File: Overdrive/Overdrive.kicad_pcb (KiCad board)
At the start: 2 copper layers, 60 x 110 mm, 50 parts, among them J1 IN, J2 DC IN, J3 OUT, Q1 MMBT2222A, Q2 MMBT2222A, SW1 SW_SPDT, U1 TL072

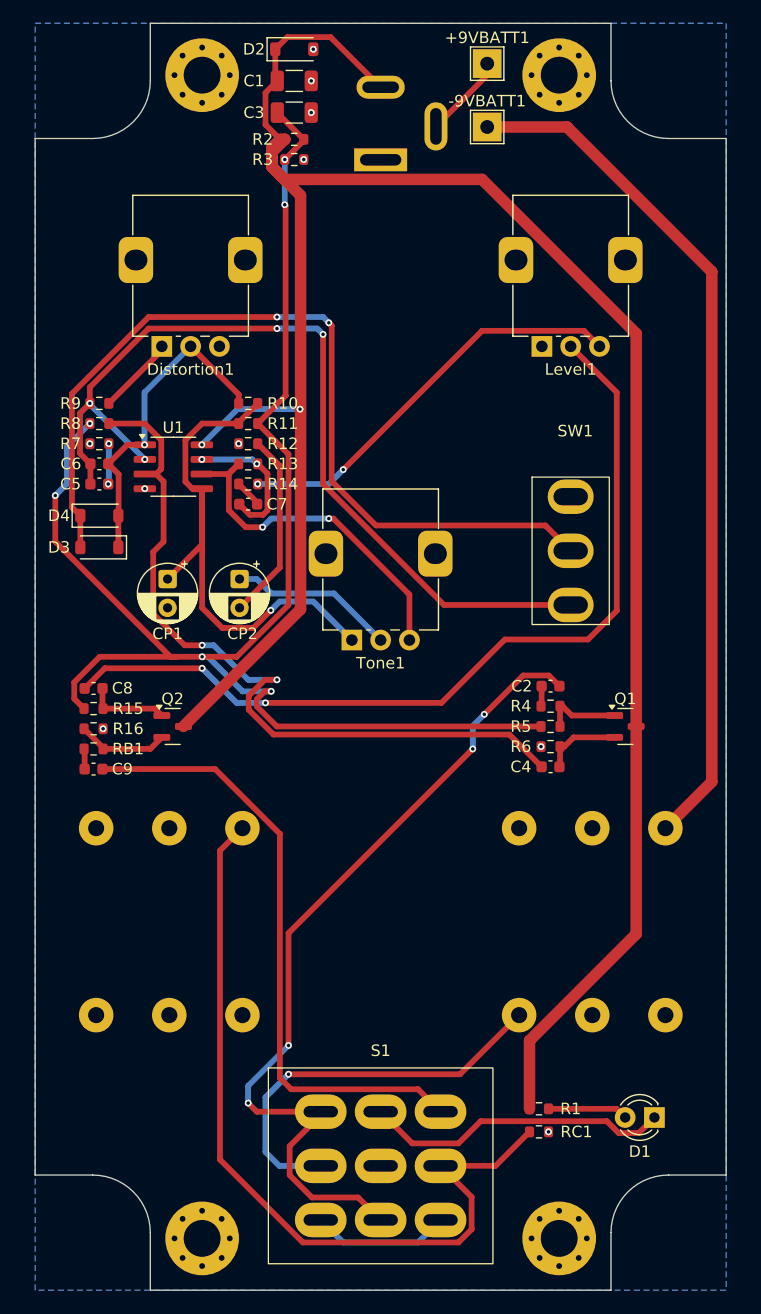
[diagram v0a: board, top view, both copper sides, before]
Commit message: done PCB layout
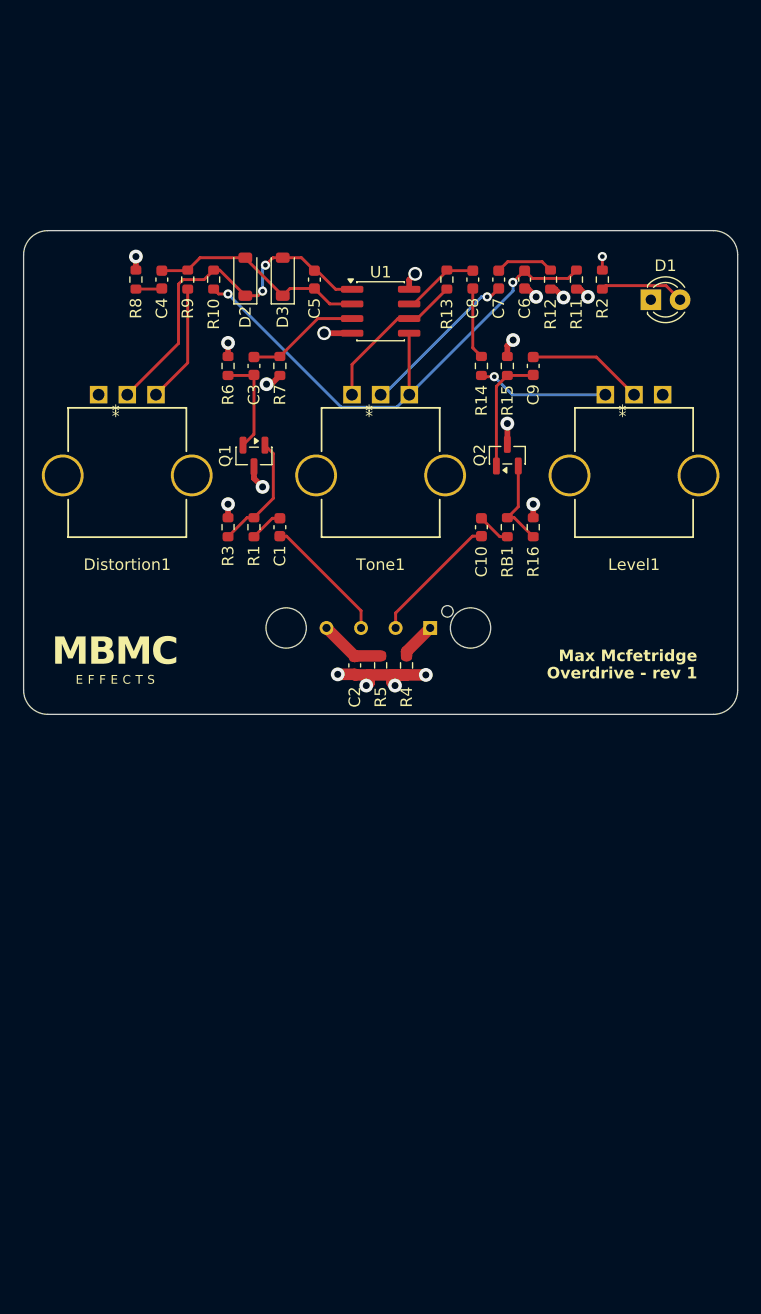
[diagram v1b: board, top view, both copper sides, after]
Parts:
- removed +9VBATT1: 9V Batt +ve, TestPoint:TestPoint_THTPad_2.5x2.5mm_Drill1.2mm
- removed -9VBATT1: 9V Batt -ve, TestPoint:TestPoint_THTPad_2.5x2.5mm_Drill1.2mm
- removed CP1, CP2: 220nF, Capacitor_THT:CP_Radial_D5.0mm_P2.50mm
- removed D4: 1N4148W, Diode_SMD:D_SOD-123
- removed H1, H2, H3, H4: MountingHole, MountingHole:MountingHole_3.2mm_M3_Pad_Via
- removed J2: DC IN, Connector_BarrelJack:BarrelJack_GCT_DCJ200-10-A_Horizontal
- removed J3: OUT, Connector_Audio:Jack_6.35mm_Neutrik_NMJ6HFD2_Horizontal
- removed RC1: 10k, Resistor_SMD:R_0603_1608Metric
- removed S1: Foot Switch, Button_Switch_THT:3PDT Foot Switch
- removed SW1: SW_SPDT, Button_Switch_THT:spdt switch custom
- added C10: 10uF, Capacitor_SMD:C_0603_1608Metric, F.Cu at (158.8, 83.8)
- C1: value 100uF -> 20nF; footprint Capacitor_SMD:C_1206_3216Metric -> Capacitor_SMD:C_0603_1608Metric
- C2: value 20nF -> 47uF
- C3: value 47uF -> 1uF; footprint Capacitor_SMD:C_1206_3216Metric -> Capacitor_SMD:C_0603_1608Metric
- C4: value 1uF -> 47nF
- C5: value 47nF -> 47pF
- C6: value 47pF -> 220nF
- C7: value 1uF -> 220nF
- C8: value 100nF -> 1uF
- C9: value 10uF -> 100nF
- Distortion1, Level1, Tone1: footprint Potentiometer_THT:Potentiometer_RK097_Single_Vertical -> PTV09A-4020F-A504:POT_PTV09A-4020F_BRN
- J1: value IN -> 303C-321018-30-04; footprint Connector_Audio:Jack_6.35mm_Neutrik_NMJ6HFD2_Horizontal -> 303C-321018-30-04:ATTEND_303C-321018-30-04
- R1: value 470R -> 1k
- R12: value 220 -> 220R
- R2: value 10K -> 470R
- R3: value 10K -> 510k
- R4: value 1k -> 10K
- R5: value 510k -> 10K
- R7: value 4.7k -> 10k
- R8: value 10k -> 4.7k
- moved D1 71.0 mm to (173.5, 64.0), turned to 0 degrees
- moved R1 56.2 mm to (139.0, 83.8), turned to 90 degrees
- moved C4 54.1 mm to (131.0, 62.2), turned to 90 degrees
- moved C9 51.8 mm to (163.2, 69.8), turned to -90 degrees
- moved C8 48.4 mm to (158.0, 62.2), turned to -90 degrees
- moved R15 46.6 mm to (161.0, 69.8), turned to -90 degrees
- moved R6 43.3 mm to (136.8, 69.8), turned to -90 degrees
- moved R16 42.0 mm to (163.2, 83.8), turned to 90 degrees
- moved RB1 40.8 mm to (161.0, 83.8), turned to 90 degrees
- moved C6 40.2 mm to (162.5, 62.2), turned to 90 degrees
- moved Q1 39.9 mm to (139.0, 77.6), turned to -90 degrees
- moved C1 38.8 mm to (141.2, 83.8), turned to 90 degrees
- moved Q2 37.4 mm to (161.0, 77.5), turned to 90 degrees
- moved J1 35.7 mm to (150.0, 92.5), turned to 180 degrees
- moved R3 32.4 mm to (136.8, 83.8), turned to 90 degrees
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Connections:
- C1 pad 1: +9V -> FX_IN
- C1 pad 2: GND -> Net-(C1-Pad2)
- C2 pad 1: Wet In -> +4.5V
- C2 pad 2: Net-(C2-Pad2) -> GND
- C3 pad 1: +4.5V -> Net-(Q1-E)
- C3 pad 2: GND -> Net-(C3-Pad2)
- C4 pad 1: Net-(Q1-E) -> Net-(C4-Pad1)
- C4 pad 2: Net-(C4-Pad2) -> Net-(D2-A)
- C5 pad 1: Net-(C5-Pad1) -> Net-(D2-A)
- C5 pad 2: Net-(SW1-C) -> Net-(D2-K)
- C6 pad 1: Net-(SW1-C) -> GND
- C6 pad 2: Net-(D3-K) -> Net-(C6-Pad2)
- C8 pad 2: Net-(Q2-B) -> Net-(C8-Pad2)
- C9 pad 2: Wet Out -> Net-(Q2-B)
- D1 pad 1: Net-(D1-K) -> GND
- D2 pad 1: +9V -> Net-(D2-K)
- D2 pad 2: GND -> Net-(D2-A)
- D3 pad 1: Net-(D3-K) -> Net-(D2-A)
- D3 pad 2: Net-(D3-A) -> Net-(D2-K)
- Distortion1 pad 2: Net-(D3-K) -> Net-(D2-K)
- Level1 pad 2: Net-(C8-Pad1) -> Net-(C9-Pad1)
- R1 pad 1: Net-(D1-A) -> Net-(C1-Pad2)
- R1 pad 2: +9V -> Net-(Q1-B)
- R10 pad 1: Net-(D3-K) -> Net-(D2-K)
- R10 pad 2: Net-(CP1-Pad1) -> Net-(C6-Pad2)
- R11 pad 1: Net-(CP1-Pad1) -> Net-(C6-Pad2)
- R12 pad 2: Net-(CP2-Pad2) -> Net-(C7-Pad2)
- R13 pad 2: Net-(C7-Pad1) -> Net-(C8-Pad1)
- R14 pad 1: Net-(C7-Pad2) -> Net-(C8-Pad2)
- R2 pad 2: +4.5V -> Net-(D1-A)
- R3 pad 1: +4.5V -> Net-(Q1-B)
- R3 pad 2: GND -> +4.5V
- R4 pad 1: Net-(C2-Pad2) -> +9V
- R4 pad 2: Net-(Q1-B) -> +4.5V
- R5 pad 1: Net-(Q1-B) -> +4.5V
- R5 pad 2: +4.5V -> GND
- R7 pad 1: GND -> +4.5V
- R7 pad 2: Net-(C5-Pad1) -> Net-(C3-Pad2)
- R8 pad 1: +4.5V -> GND
- R8 pad 2: Net-(C4-Pad2) -> Net-(C4-Pad1)
- R9 pad 1: Net-(SW1-C) -> Net-(Distortion1-Pad1)
- R9 pad 2: Net-(Distortion1-Pad1) -> Net-(D2-A)
- RB1 pad 1: Net-(C9-Pad1) -> Net-(C10-Pad1)
- Tone1 pad 1: Net-(CP1-Pad1) -> Net-(C6-Pad2)
- Tone1 pad 2: Net-(CP2-Pad1) -> Net-(C7-Pad1)
- U1 pad 1: Net-(D3-K) -> Net-(D2-K)
- U1 pad 2: Net-(SW1-C) -> Net-(D2-A)
- U1 pad 3: Net-(C4-Pad2) -> Net-(C3-Pad2)
- U1 pad 5: Net-(CP1-Pad1) -> Net-(C6-Pad2)
- U1 pad 7: Net-(C7-Pad1) -> Net-(C8-Pad1)
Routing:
- net +9V: track 201.0 -> 9.88 mm, vias 2 -> 4
- net +4.5V: track 131.4 -> 16.5 mm, vias 6 -> 8
- net Net-(SW1-C): track 77.4 -> 0.00 mm, vias 4 -> 0
- net Net-(D3-A): track 76.0 -> 0.00 mm, vias 2 -> 0
- net Net-(-9VBATT1-Pad1): track 74.7 -> 0.00 mm
- net Wet In: track 73.0 -> 0.00 mm, vias 4 -> 0
- net Guitar Out: track 70.5 -> 0.00 mm
- net Net-(C8-Pad1): track 76.1 -> 6.81 mm, vias 2 -> 0
- net Net-(C4-Pad2): track 66.9 -> 0.00 mm, vias 2 -> 0
- net Wet Out: track 54.1 -> 0.00 mm
- net Net-(CP1-Pad1): track 48.3 -> 0.00 mm, vias 1 -> 0
- net Net-(C6-Pad2): track 0.00 -> 47.0 mm, vias 0 -> 2
- net Guitar In: track 35.0 -> 0.00 mm, vias 1 -> 0
- net Net-(D2-K): track 0.00 -> 31.6 mm, vias 0 -> 2
- net Net-(D3-K): track 28.3 -> 0.00 mm, vias 1 -> 0
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- added copper zone on In2.Cu, net +4.5V
- added copper zone on In2.Cu, net +9V
- added copper zone on In1.Cu, net GND
- removed copper zone on B.Cu, net GND
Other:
- board size 60 x 110 mm -> 62 x 42 mm
- copper layers 2 -> 4
- board text added: "Max Mcfetridge"
- board text added: "Overdrive - rev 1"
